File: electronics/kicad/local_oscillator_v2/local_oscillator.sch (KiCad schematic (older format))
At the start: 20 parts, among them P1 TestPoint:TestPoint_Pad_1.5x1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, P2 TestPoint:TestPoint_Pad_1.5x1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, P3 TestPoint:TestPoint_Pad_1.5x1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, P4 TestPoint:TestPoint_Pad_1.5x1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, U1 CE3520K3

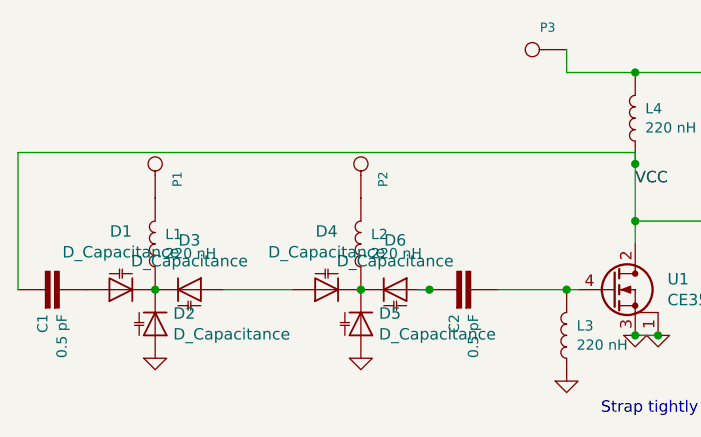
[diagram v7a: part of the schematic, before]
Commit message: Hell yeah! DC biasing
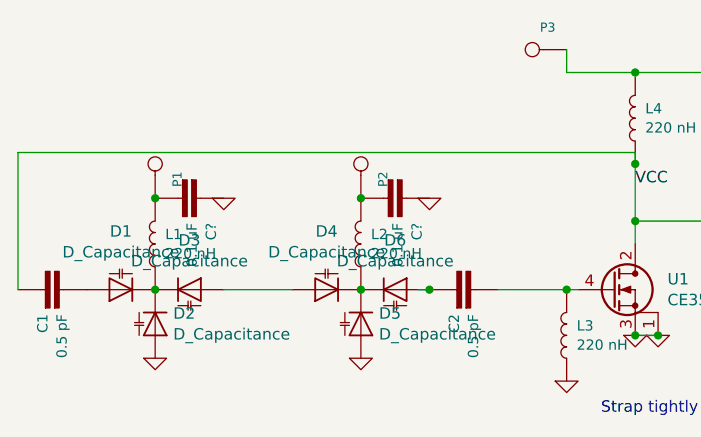
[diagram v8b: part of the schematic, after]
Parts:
- added C? (x2): 0.1 uF, 0603, symbol SparkFun-Capacitors:4.7UF0603
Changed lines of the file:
@@
 	0    -1   -1   0
 $EndComp
+$Comp
+L SparkFun-Capacitors:4.7UF0603 C?
+U 1 1 5ED6E617
+P 3650 4250
+F 0 "C?" H 3758 4395 45  0000 L CNN
+F 1 "0.1 uF" H 3758 4311 45  0000 L CNN
+F 2 "0603" H 3650 4500 20  0001 C CNN
+F 3 "" H 3650 4250 50  0001 C CNN
+F 4 "CAP-08280" V 3758 4216 60  0001 L CNN "Field4"
+	1    3650 4250
+	0    1    1    0
+$EndComp
+Connection ~ 3550 4250
+$Comp
+L SparkFun-Capacitors:4.7UF0603 C?
+U 1 1 5ED6F7F8
+P 4550 4250
+F 0 "C?" H 4658 4395 45  0000 L CNN
+F 1 "0.1 uF" H 4658 4311 45  0000 L CNN
+F 2 "0603" H 4550 4500 20  0001 C CNN
+F 3 "" H 4550 4250 50  0001 C CNN
+F 4 "CAP-08280" V 4658 4216 60  0001 L CNN "Field4"
+	1    4550 4250
+	0    1    1    0
+$EndComp
+Connection ~ 4450 4250
+$Comp
+L power:GND #PWR?
+U 1 1 5ED6FEF6
+P 4750 4250
+F 0 "#PWR?" H 4750 4250 30  0001 C CNN
+F 1 "GND" H 4750 4180 30  0001 C CNN
+F 2 "" H 4750 4250 50  0001 C CNN
+F 3 "" H 4750 4250 50  0001 C CNN
+	1    4750 4250
+	1    0    0    -1
+$EndComp
+$Comp
+L power:GND #PWR?
+U 1 1 5ED70604
+P 3850 4250
+F 0 "#PWR?" H 3850 4250 30  0001 C CNN
+F 1 "GND" H 3850 4180 30  0001 C CNN
+F 2 "" H 3850 4250 50  0001 C CNN
+F 3 "" H 3850 4250 50  0001 C CNN
+	1    3850 4250
+	1    0    0    -1
+$EndComp
 $EndSCHEMATC
